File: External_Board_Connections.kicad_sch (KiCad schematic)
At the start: 16 parts, among them J1 Conn_01x04, J10 Conn_01x02, J11 Conn_01x06, J12 Conn_01x02, J13 Conn_01x02, J14 Conn_01x02, J15 Conn_01x02, J19 Conn_01x01_Socket, J20 Conn_01x01_Socket, J21 Conn_01x01_Socket, J22 Conn_01x01_Socket, J6 Conn_02x04_Odd_Even, J7 Conn_02x04_Odd_Even, J8 Conn_02x04_Odd_Even, J9 Conn_02x04_Odd_Even

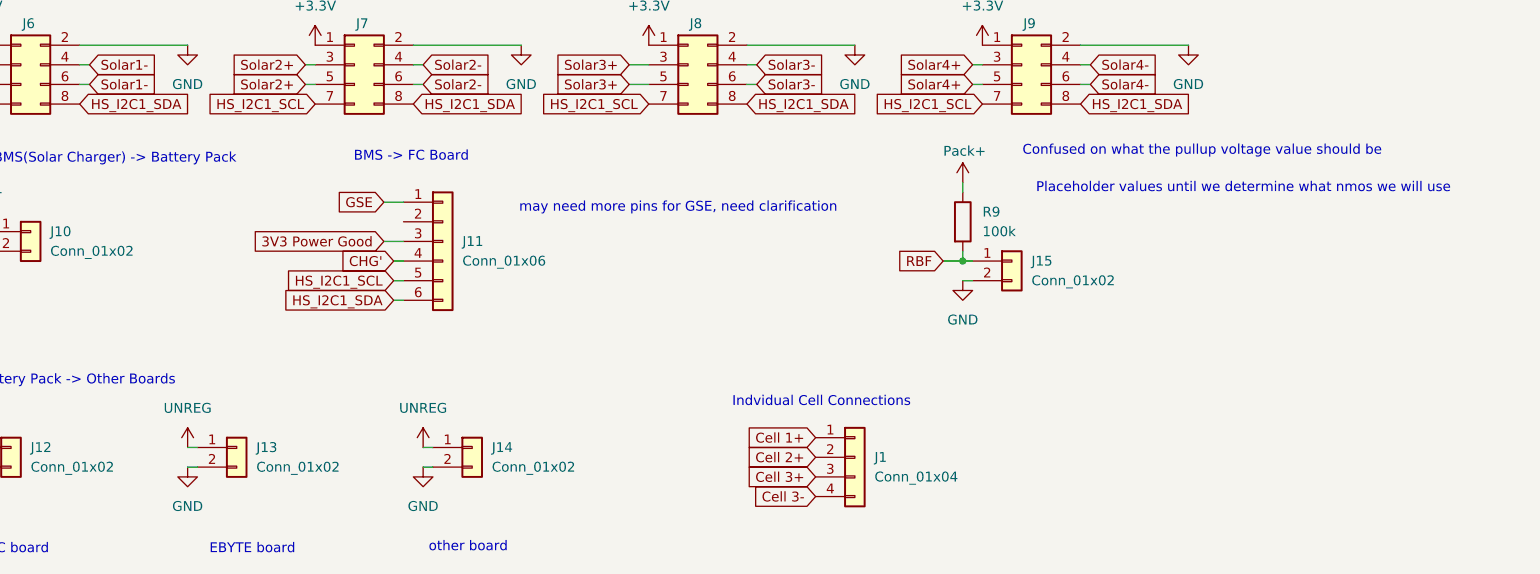
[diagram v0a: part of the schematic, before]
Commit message: Inhibit
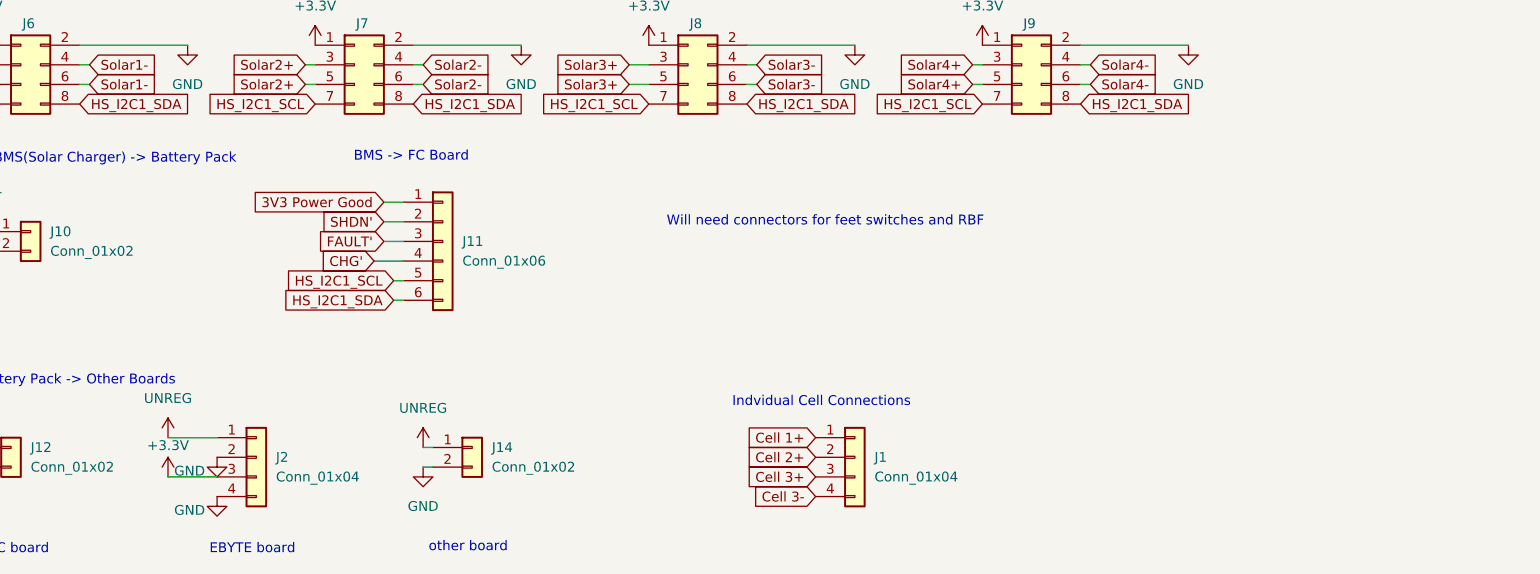
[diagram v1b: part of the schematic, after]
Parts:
- removed J13, J15: Conn_01x02, symbol Connector_Generic:Conn_01x02
- removed R9: 100k, symbol Device:R
- added J2: Conn_01x04, symbol Connector_Generic:Conn_01x04
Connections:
- net GSE is gone; now on net 3V3 Power Good: J11.1 (Pin_1)
- net +3.3V: now also J2.3 (Pin_3)
- net 3V3 Power Good: no longer J11.3 (Pin_3)
- net GND: now also J2.2 (Pin_2), J2.4 (Pin_4)
- net UNREG: now also J2.1 (Pin_1)
- net SHDN': now reaches J11.2 (Pin_2)
- new net FAULT': J11.3 (Pin_3)
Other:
- note added: "Will need connectors for feet switches and RBF"
- note removed: "Confused on what the pullup voltage value should be"
- note removed: "Placeholder values until we determine what nmos we will use"
- note removed: "may need more pins for GSE, need clarification"
